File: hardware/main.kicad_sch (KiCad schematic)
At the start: 1 part, among them U2 RK3328

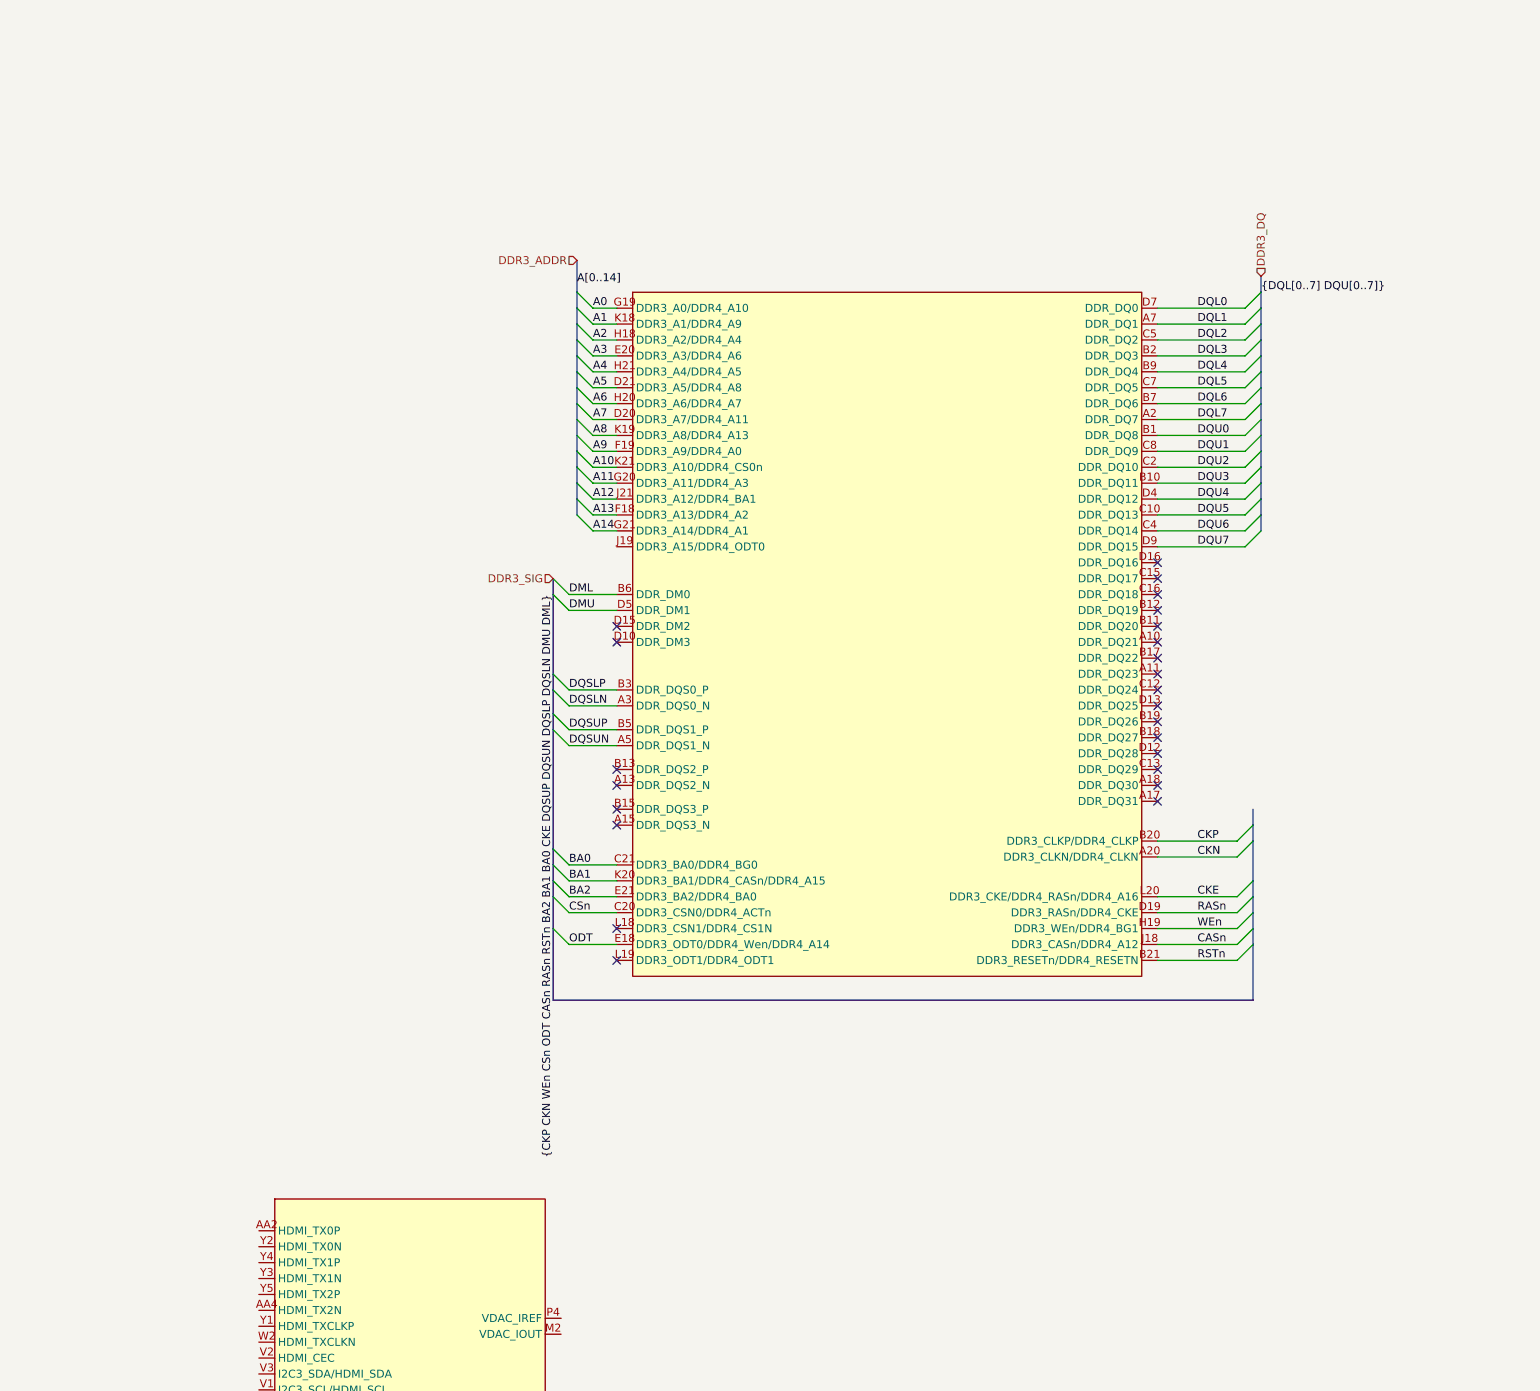
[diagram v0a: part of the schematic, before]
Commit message: stuff
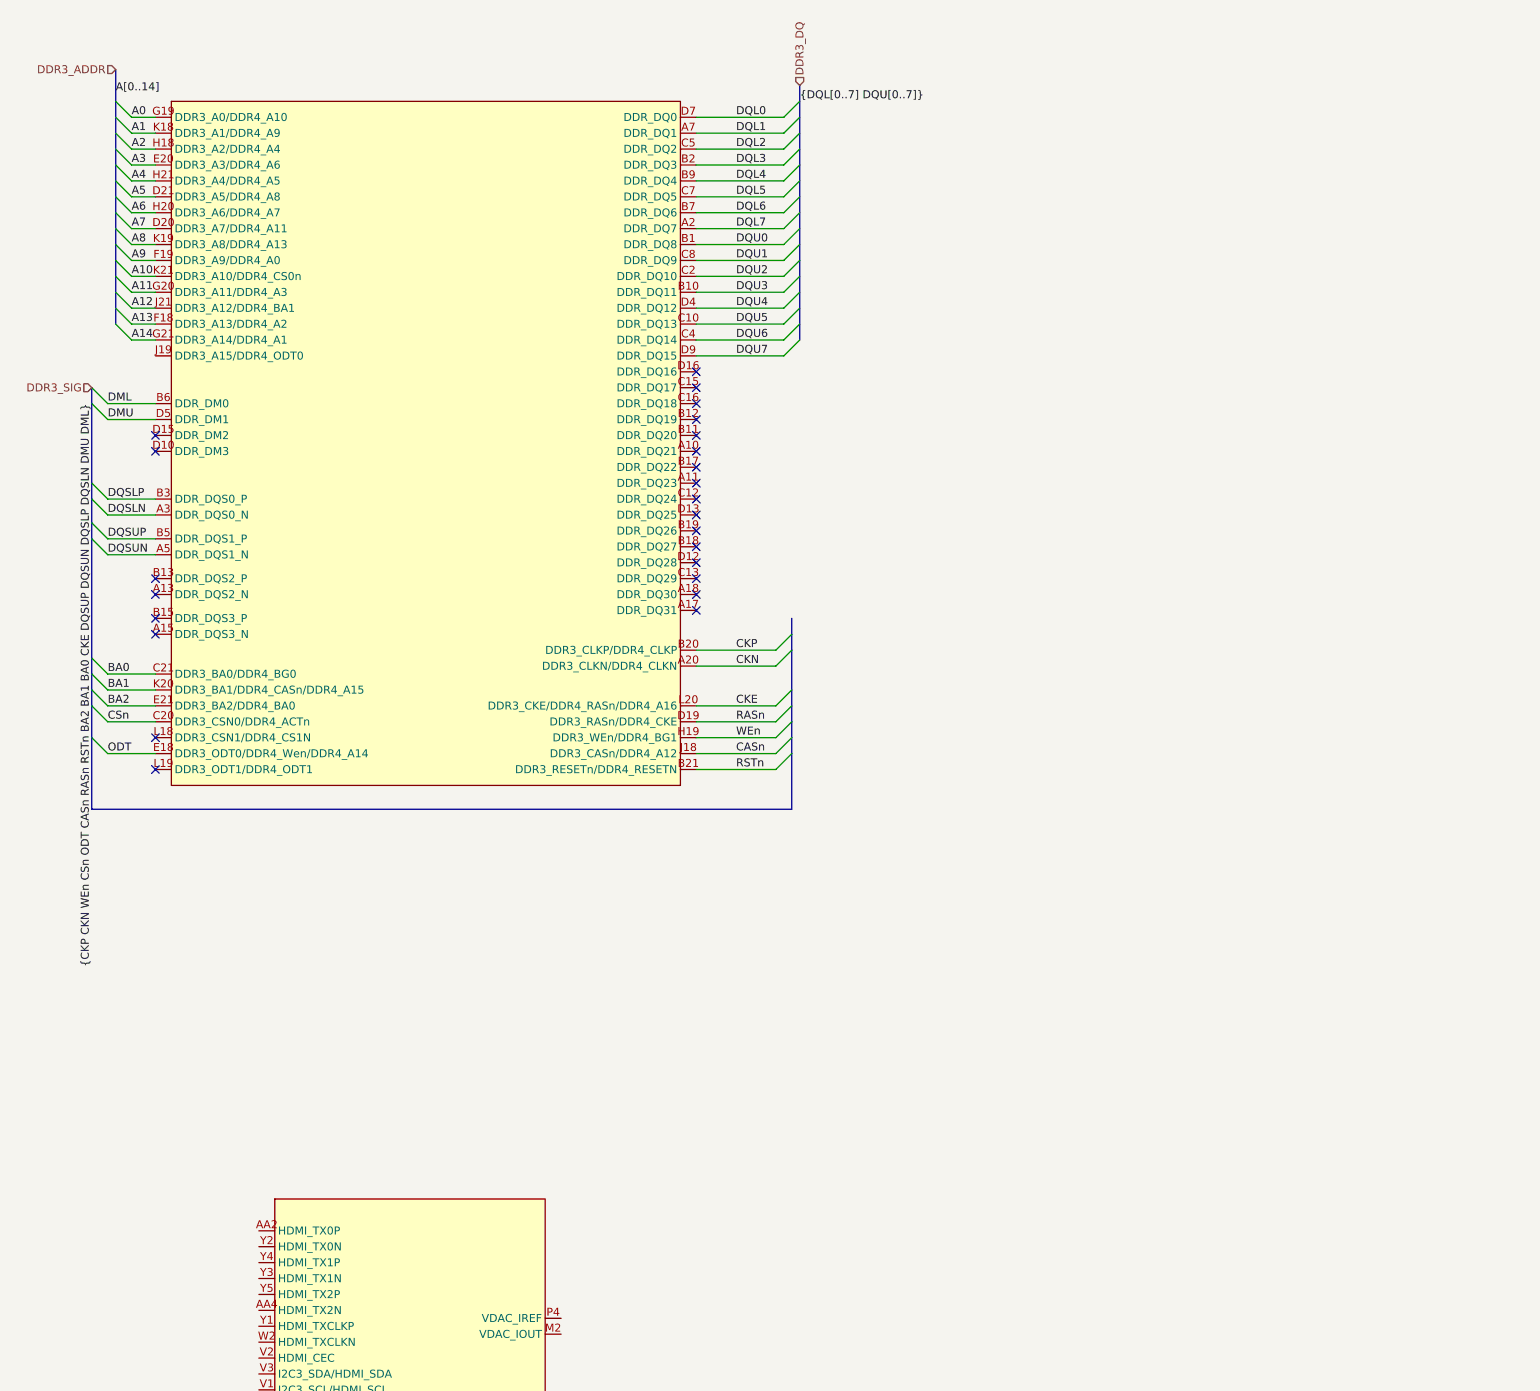
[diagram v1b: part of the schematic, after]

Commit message: stuff
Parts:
- added R13: R, symbol Device:R
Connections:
- net PHY_RXN: now reaches U2.AA8 (FEPHY_RXN)
- net PHY_TXN: now reaches U2.AA9 (FEPHY_TXN)
- net at U2.V7 (FEPHY_EXTRES): now also R13.1
- net PHY_RXP: now reaches U2.Y8 (FEPHY_RXP)
- net PHY_TXP: now reaches U2.Y9 (FEPHY_TXP)
- net SD_DAT3: now reaches U2.AA13 (GPIO1_A3/SDMMC0_D3/JTAG_TMS)
- net SD_DAT0: now reaches U2.U10 (GPIO1_A0/SDMMC0_D0/UART2_TX_M0)
- net SD_DETN: now reaches U2.V10 (GPIO1_A5/SDMMC0_DETN)
- net SD_DAT1: now reaches U2.W11 (GPIO1_A1/SDMMC0_D1/UART2_RX_M0)
- net SD_CLK: now reaches U2.W12 (GPIO1_A6/SDMMC0_CLK/TEST_CLK0)
- net SD_DAT2: now reaches U2.W13 (GPIO1_A2/SDMMC0_D2/JTAG_TCK)
- net SD_CMD: now reaches U2.Y13 (GPIO1_A4/SDMMC0_CMD)
- new net GND: R13.2
- new net PHY_DATA_LED: U2.R17 (GPIO2_D1/I2C0_SDA/FEPHY_LED_DATA_M1)
- new net PHY_LINK_LED: U2.P17 (GPIO2_D0/I2C0_SCL/FEPHY_LED_LINK_M1)
